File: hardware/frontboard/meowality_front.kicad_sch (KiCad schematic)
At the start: 58 parts

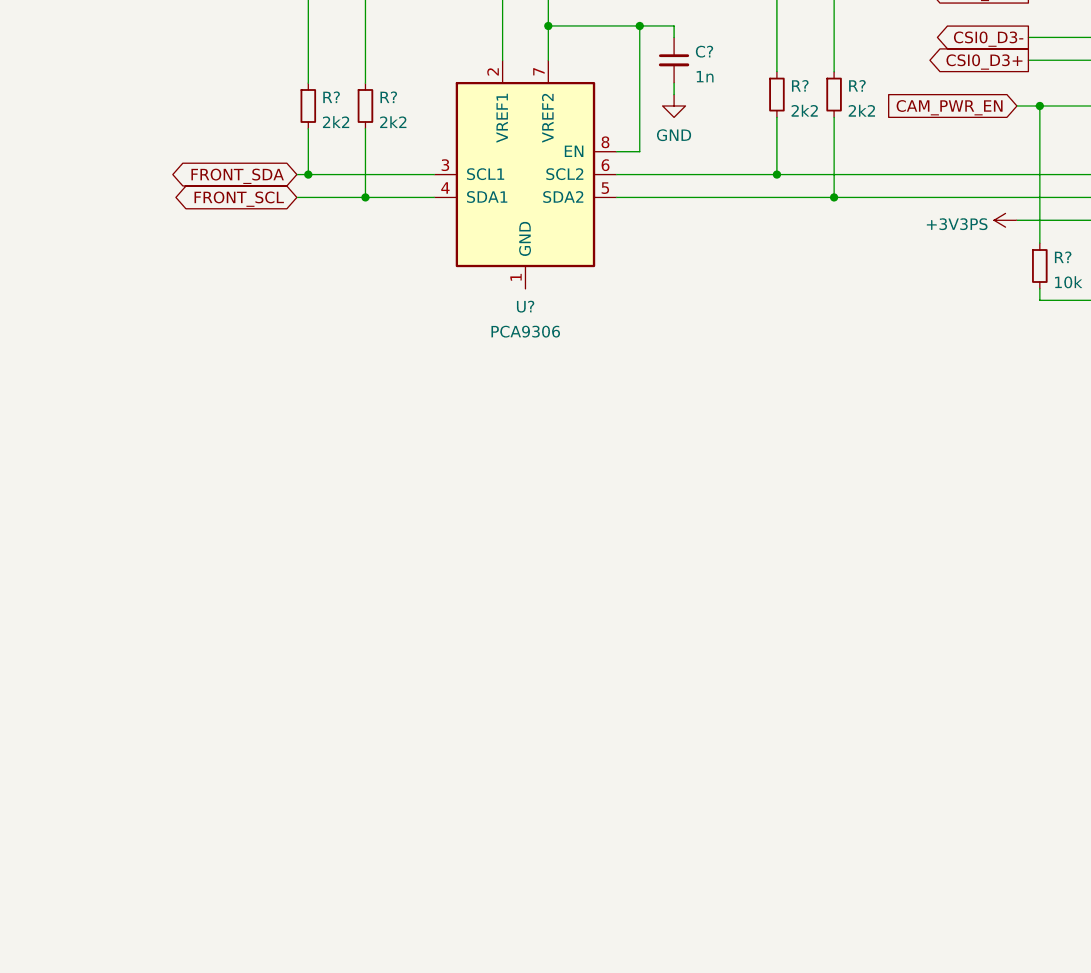
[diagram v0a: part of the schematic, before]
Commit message: Add IMU
Signed-off-by: gatecat <gatecat@ds0.me>
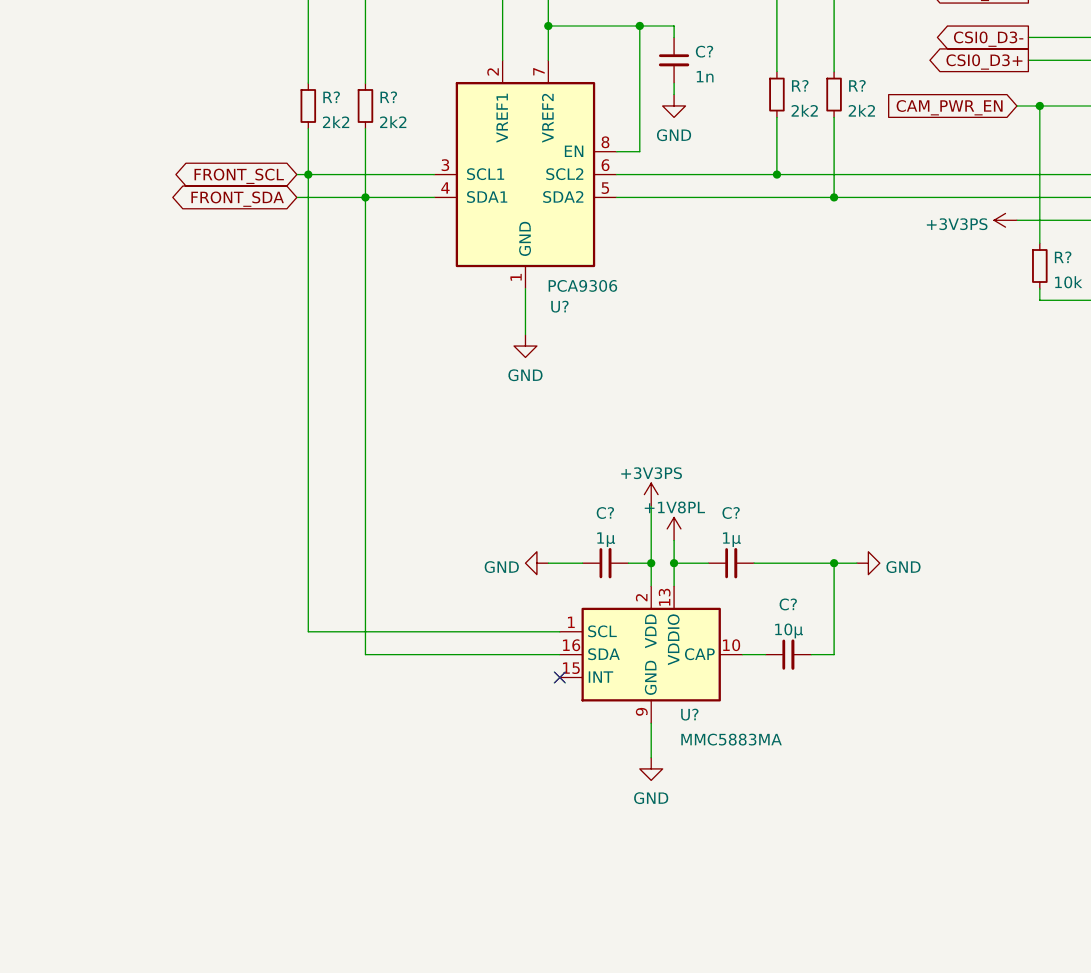
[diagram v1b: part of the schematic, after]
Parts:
- added C? (x2): 1µ, symbol Device:C_Small
- added C?: 10µ, symbol Device:C_Small
- added U?: MMC5883MA, Package_LGA:LGA-16_3x3mm_P0.5mm, symbol Sensor_Magnetic:MMC5883MA
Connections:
- net +1V8PL: now also C?.1, U?.13 (VDDIO)
- net +3V3PS: now also C?.2, U?.2 (VDD)
- net FRONT_SCL: now also R?.2, U?.3 (SCL1), U?.1 (SCL); no longer R?.2, U?.4 (SDA1)
- net FRONT_SDA: now also R?.2, U?.4 (SDA1), U?.16 (SDA); no longer R?.2, U?.3 (SCL1)
- net GND: now also U?.1 (GND), C?.1, C?.2, C?.2, U?.11 (GND), U?.9 (GND)
- new net: C?.1, U?.10 (CAP)
- no-connect marks 42 -> 43
